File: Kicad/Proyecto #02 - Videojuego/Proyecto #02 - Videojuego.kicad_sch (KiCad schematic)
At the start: 16 parts

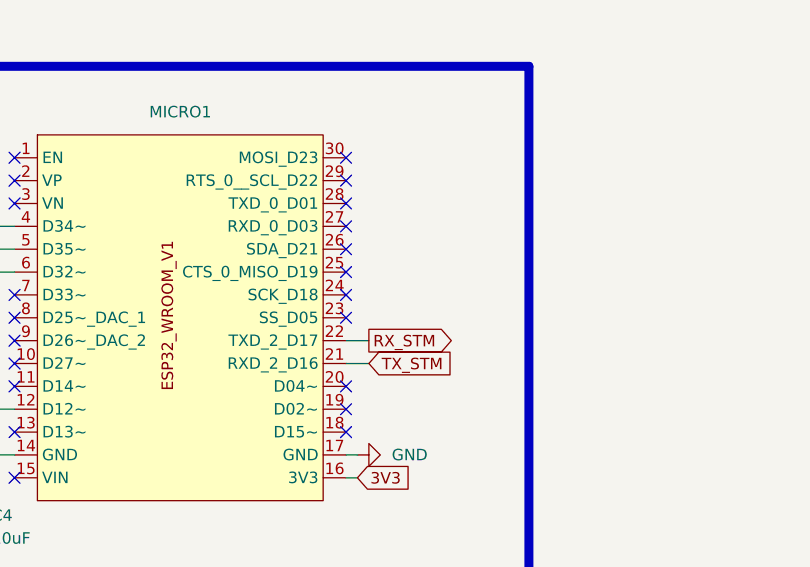
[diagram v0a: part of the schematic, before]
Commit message: A
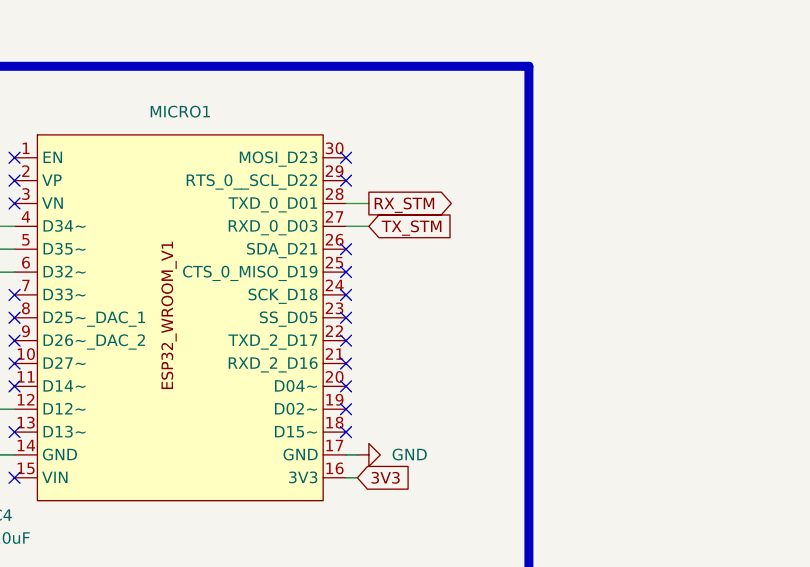
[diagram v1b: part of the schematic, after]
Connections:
- net RX_STM: now also MICRO1.28 (TXD_0_D01); no longer MICRO1.22 (TXD_2_D17)
- net TX_STM: now also MICRO1.27 (RXD_0_D03); no longer MICRO1.21 (RXD_2_D16)
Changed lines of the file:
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@@
-	)
-	(no_connect
-		(at 340.36 152.4)
 	)
 	(no_connect
@@
 	)
 	(no_connect
+		(at 340.36 170.18)
+	)
+	(no_connect
 		(at 193.04 54.61)
 	)
@@
 	)
 	(no_connect
+		(at 340.36 167.64)
+	)
+	(no_connect
 		(at 303.53 152.4)
 	)
@@
 	)
 	(no_connect
-		(at 340.36 154.94)
-	)
-	(no_connect
 		(at 193.04 50.8)
 	)
@@
 	(wire
 		(pts
-			(xy 340.36 167.64) (xy 342.9 167.64)
-		)
-		(stroke
-			(width 0)
-			(type default)
-		)
-	)
-	(wire
-		(pts
 			(xy 198.12 175.26) (xy 198.12 205.74)
 		)
@@
 	(wire
 		(pts
+			(xy 340.36 154.94) (xy 342.9 154.94)
+		)
+		(stroke
+			(width 0)
+			(type default)
+		)
+	)
+	(wire
+		(pts
 			(xy 205.74 152.4) (xy 205.74 213.36)
 		)
@@
 	(wire
 		(pts
+			(xy 340.36 152.4) (xy 342.9 152.4)
+		)
+		(stroke
+			(width 0)
+			(type default)
+		)
+	)
+	(wire
+		(pts
 			(xy 349.25 85.09) (xy 349.25 87.63)
 		)
@@
 		(pts
 			(xy 156.21 215.9) (xy 156.21 243.84)
-		)
-		(stroke
-			(width 0)
-			(type default)
-		)
-	)
-	(wire
-		(pts
-			(xy 340.36 170.18) (xy 342.9 170.18)
 		)
 		(stroke
@@
 	(global_label "RX_STM"
 		(shape output)
-		(at 342.9 167.64 0)
+		(at 342.9 152.4 0)
 		(fields_autoplaced yes)
 		(effects
@@
 		)
 		(property "Intersheetrefs" "${INTERSHEET_REFS}"
-			(at 352.8703 167.64 0)
+			(at 352.8703 152.4 0)
 			(effects
 				(font
@@
 	(global_label "TX_STM"
 		(shape input)
-		(at 342.9 170.18 0)
+		(at 342.9 154.94 0)
 		(fields_autoplaced yes)
 		(effects
@@
 		)
 		(property "Intersheetrefs" "${INTERSHEET_REFS}"
-			(at 352.673 170.18 0)
+			(at 352.673 154.94 0)
 			(effects
 				(font

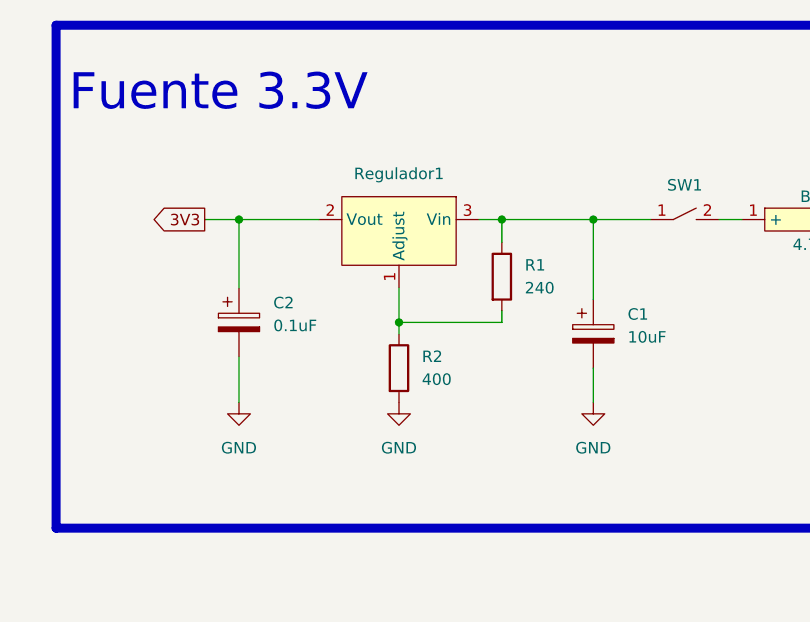
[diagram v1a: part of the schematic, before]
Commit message: A
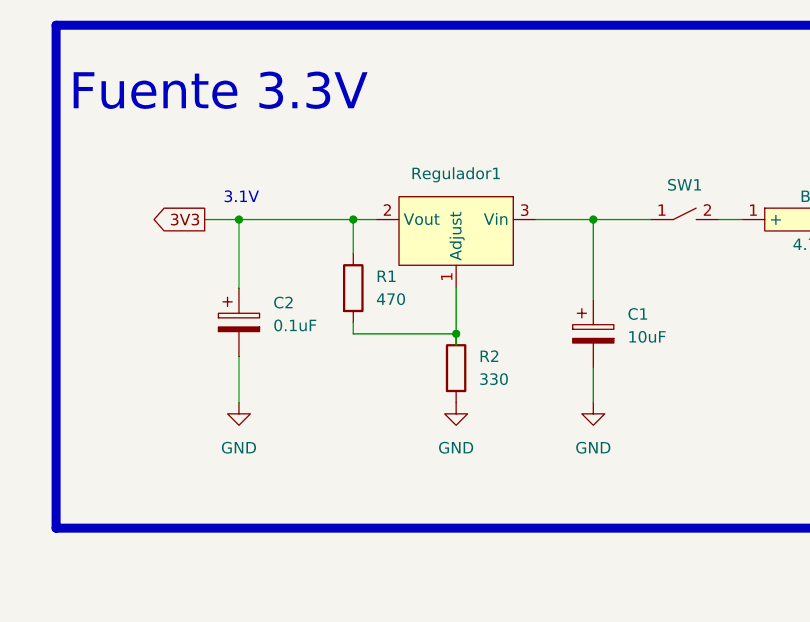
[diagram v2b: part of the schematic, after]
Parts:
- R1: value 240 -> 470
- R2: value 400 -> 330
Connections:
- net 3V3: now also R1.1
- net at C1.1, Regulador1.3 (Vin), SW1.1: no longer R1.1
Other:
- note added: "3.1V"
- moved on the sheet: R1, R2, Regulador1
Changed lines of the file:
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@@
-	)
-	(junction
-		(at 293.37 96.52)
-		(diameter 0)
-		(color 0 0 0 0)
 	)
 	(junction
@@
 	)
 	(junction
-		(at 297.18 175.26)
+		(at 299.72 97.79)
 		(diameter 0)
 		(color 0 0 0 0)
 	)
 	(junction
-		(at 304.8 85.09)
+		(at 297.18 175.26)
 		(diameter 0)
 		(color 0 0 0 0)
@@
 		(color 0 0 0 0)
 	)
+	(junction
+		(at 288.29 85.09)
+		(diameter 0)
+		(color 0 0 0 0)
+	)
 	(no_connect
 		(at 193.04 115.57)
@@
 	(wire
 		(pts
-			(xy 304.8 96.52) (xy 304.8 95.25)
-		)
-		(stroke
-			(width 0)
-			(type default)
-		)
-	)
-	(wire
-		(pts
 			(xy 153.67 213.36) (xy 153.67 238.76)
 		)
@@
 	(wire
 		(pts
-			(xy 304.8 85.09) (xy 314.96 85.09)
-		)
-		(stroke
-			(width 0)
-			(type default)
-		)
-	)
-	(wire
-		(pts
 			(xy 203.2 210.82) (xy 151.13 210.82)
 		)
@@
 	(wire
 		(pts
-			(xy 293.37 96.52) (xy 304.8 96.52)
-		)
-		(stroke
-			(width 0)
-			(type default)
-		)
-	)
-	(wire
-		(pts
 			(xy 115.57 233.68) (xy 118.11 233.68)
 		)
@@
 	(wire
 		(pts
-			(xy 293.37 92.71) (xy 293.37 96.52)
+			(xy 299.72 92.71) (xy 299.72 97.79)
 		)
 		(stroke
@@
 	(wire
 		(pts
+			(xy 288.29 85.09) (xy 290.83 85.09)
+		)
+		(stroke
+			(width 0)
+			(type default)
+		)
+	)
+	(wire
+		(pts
 			(xy 328.93 85.09) (xy 331.47 85.09)
 		)
@@
 	(wire
 		(pts
-			(xy 293.37 96.52) (xy 293.37 97.79)
-		)
-		(stroke
-			(width 0)
-			(type default)
-		)
-	)
-	(wire
-		(pts
 			(xy 193.04 186.69) (xy 194.31 186.69)
 		)
@@
 	(wire
 		(pts
-			(xy 302.26 85.09) (xy 304.8 85.09)
+			(xy 308.61 85.09) (xy 314.96 85.09)
 		)
 		(stroke
@@
 	(wire
 		(pts
+			(xy 288.29 97.79) (xy 299.72 97.79)
+		)
+		(stroke
+			(width 0)
+			(type default)
+		)
+	)
+	(wire
+		(pts
 			(xy 203.2 160.02) (xy 203.2 210.82)
 		)
@@
 	(wire
 		(pts
+			(xy 288.29 97.79) (xy 288.29 96.52)
+		)
+		(stroke
+			(width 0)
+			(type default)
+		)
+	)
+	(wire
+		(pts
+			(xy 299.72 99.06) (xy 299.72 97.79)
+		)
+		(stroke
+			(width 0)
+			(type default)
+		)
+	)
+	(wire
+		(pts
 			(xy 67.31 167.64) (xy 69.85 167.64)
 		)
@@
 	(wire
 		(pts
+			(xy 288.29 88.9) (xy 288.29 85.09)
+		)
+		(stroke
+			(width 0)
+			(type default)
+		)
+	)
+	(wire
+		(pts
 			(xy 64.77 220.98) (xy 118.11 220.98)
 		)
@@
 	(wire
 		(pts
-			(xy 304.8 87.63) (xy 304.8 85.09)
-		)
-		(stroke
-			(width 0)
-			(type default)
-		)
-	)
-	(wire
-		(pts
 			(xy 68.58 213.36) (xy 118.11 213.36)
 		)
@@
 	(wire
 		(pts
-			(xy 275.59 85.09) (xy 284.48 85.09)
+			(xy 275.59 85.09) (xy 288.29 85.09)
 		)
 		(stroke
@@
 		(fill
 			(type none)
+		)
+	)
+	(text "3.1V\n"
+		(exclude_from_sim no)
+		(at 275.844 82.804 0)
+		(effects
+			(font
+				(size 1.27 1.27)
+			)
 		)
 	)
@@
 	(symbol
 		(lib_id "Device:R")
-		(at 304.8 91.44 0)
+		(at 288.29 92.71 0)
 		(unit 1)
 		(exclude_from_sim no)
@@
 		(fields_autoplaced yes)
 		(property "Reference" "R1"
-			(at 307.34 90.17 0)
+			(at 290.83 91.44 0)
 			(effects
 				(font
@@
 			)
 		)
-		(property "Value" "240"
-			(at 307.34 92.71 0)
+		(property "Value" "470"
+			(at 290.83 93.98 0)
 			(effects
 				(font
@@
 		)
 		(property "Footprint" ""
-			(at 303.022 91.44 90)
+			(at 286.512 92.71 90)
 			(effects
 				(font
@@
 		)
 		(property "Datasheet" "~"
-			(at 304.8 91.44 0)
+			(at 288.29 92.71 0)
 			(effects
 				(font
@@
 		)
 		(property "Description" "Resistor"
-			(at 304.8 91.44 0)
+			(at 288.29 92.71 0)
 			(effects
 				(font
@@
 	(symbol
 		(lib_id "Device:R")
-		(at 293.37 101.6 0)
+		(at 299.72 101.6 0)
 		(unit 1)
 		(exclude_from_sim no)
@@
 		(fields_autoplaced yes)
 		(property "Reference" "R2"
-			(at 295.91 100.33 0)
+			(at 302.26 100.33 0)
 			(effects
 				(font
@@
 			)
 		)
-		(property "Value" "400"
-			(at 295.91 102.87 0)
+		(property "Value" "330"
+			(at 302.26 102.87 0)
 			(effects
 				(font
@@
 		)
 		(property "Footprint" ""
-			(at 291.592 101.6 90)
+			(at 297.942 101.6 90)
 			(effects
 				(font
@@
 		)
 		(property "Datasheet" "~"
-			(at 293.37 101.6 0)
+			(at 299.72 101.6 0)
 			(effects
 				(font
@@
 		)
 		(property "Description" "Resistor"
-			(at 293.37 101.6 0)
+			(at 299.72 101.6 0)
 			(effects
 				(font
@@
 	(symbol
 		(lib_id "power:GND")
-		(at 293.37 105.41 0)
+		(at 299.72 105.41 0)
 		(unit 1)
 		(exclude_from_sim no)
@@
 		(fields_autoplaced yes)
 		(property "Reference" "#PWR05"
-			(at 293.37 111.76 0)
+			(at 299.72 111.76 0)
 			(effects
 				(font
@@
 		)
 		(property "Value" "GND"
-			(at 293.37 110.49 0)
+			(at 299.72 110.49 0)
 			(effects
 				(font
@@
 		)
 		(property "Footprint" ""
-			(at 293.37 105.41 0)
+			(at 299.72 105.41 0)
 			(effects
 				(font
@@
 		)
 		(property "Datasheet" ""
-			(at 293.37 105.41 0)
+			(at 299.72 105.41 0)
 			(effects
 				(font
@@
 		)
 		(property "Description" "Power symbol creates a global label with name \"GND\" , ground"
-			(at 293.37 105.41 0)
+			(at 299.72 105.41 0)
 			(effects
 				(font
@@
 	(symbol
 		(lib_id "JOYSTICK_KY-023:LM317")
-		(at 293.37 81.28 0)
+		(at 299.72 81.28 0)
 		(mirror y)
 		(unit 1)
@@
 		(dnp no)
 		(property "Reference" "Regulador1"
-			(at 293.37 80.01 0)
+			(at 299.72 80.01 0)
 			(effects
 				(font
@@
 		)
 		(property "Value" "~"
-			(at 293.37 81.28 0)
+			(at 299.72 81.28 0)
 			(effects
 				(font
@@
 		)
 		(property "Footprint" ""
-			(at 293.37 81.28 0)
+			(at 299.72 81.28 0)
 			(effects
 				(font
@@
 		)
 		(property "Datasheet" ""
-			(at 293.37 81.28 0)
+			(at 299.72 81.28 0)
 			(effects
 				(font
@@
 		)
 		(property "Description" ""
-			(at 293.37 81.28 0)
-			(effects
-				(font
+			(at 299.72 81.28 0)
+			(effects
+				(font

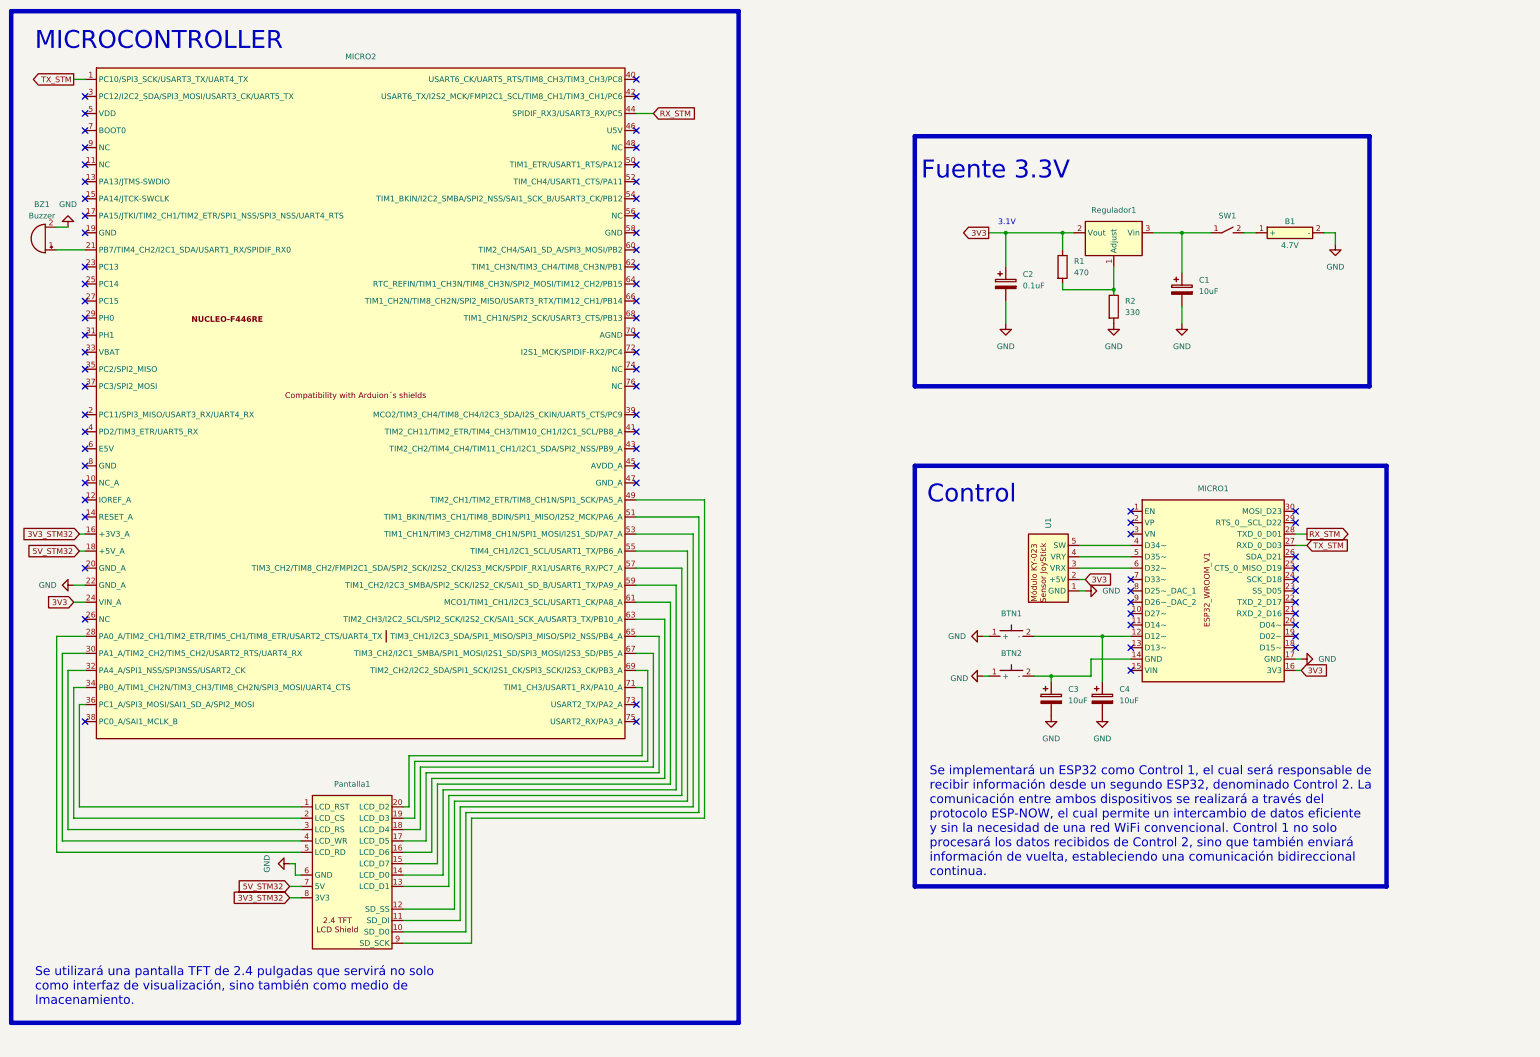
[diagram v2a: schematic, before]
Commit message: A
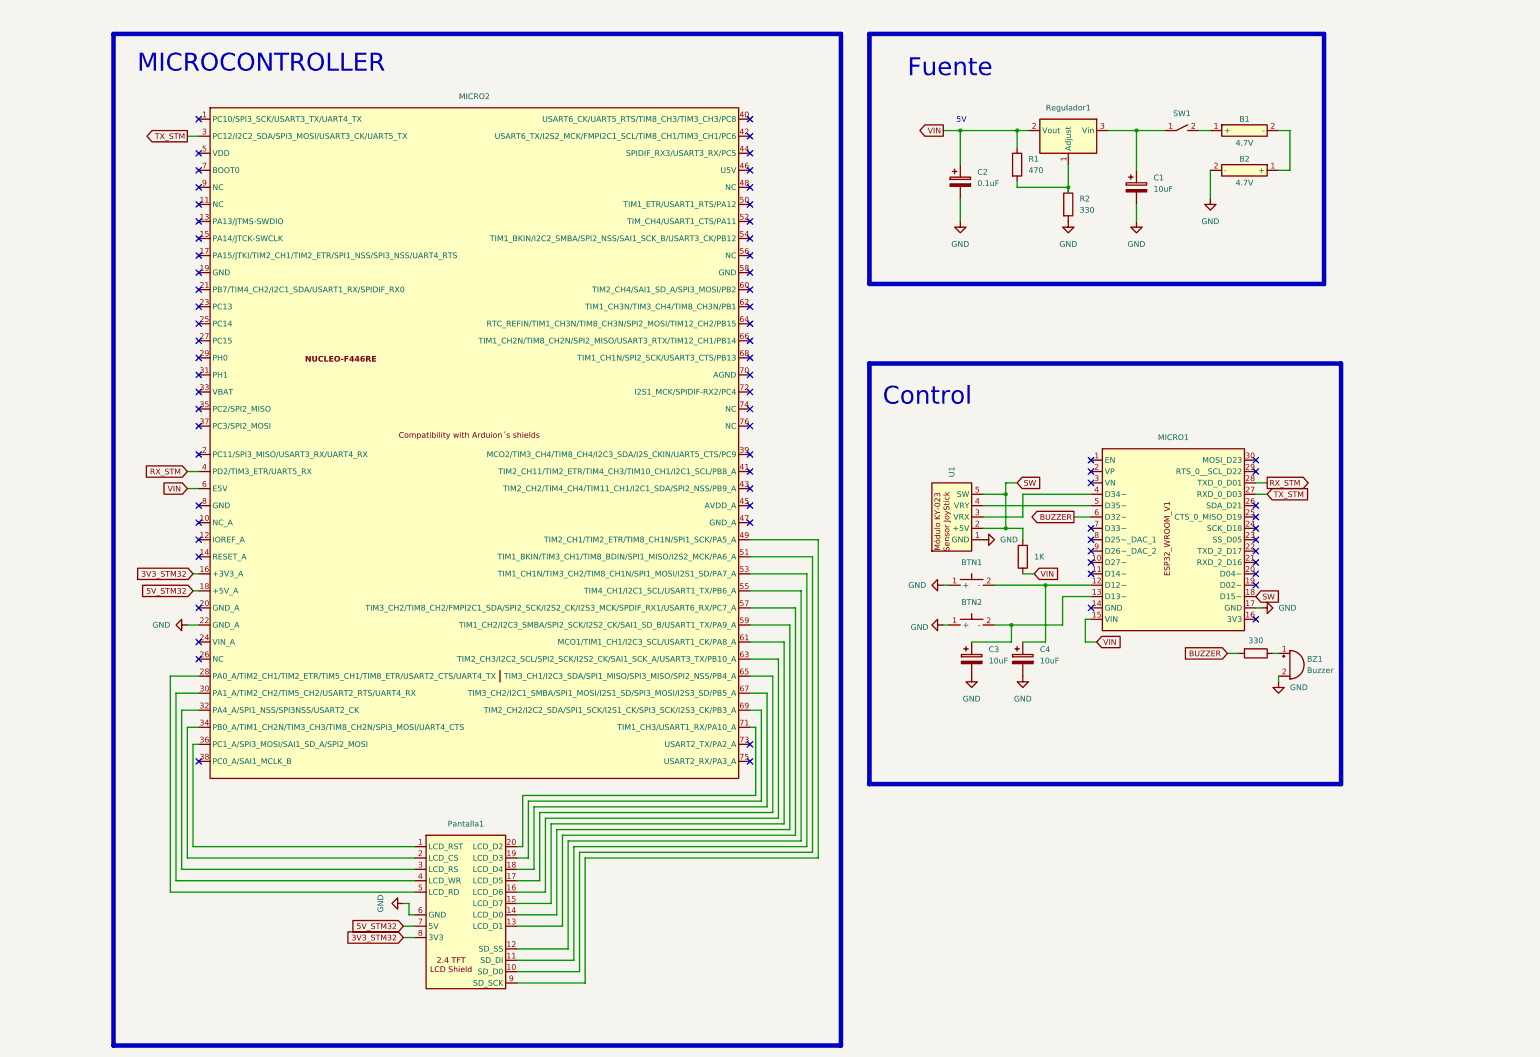
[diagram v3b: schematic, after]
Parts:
- added B2: 4.7V, symbol JOYSTICK_KY-023:Batterias
- added R3: 1K, symbol Device:R
- added R4: 330, symbol Device:R
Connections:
- net GND: now also B2.2 (-); no longer B1.2 (-)
- net RX_STM: now also MICRO2.4 (PD2/TIM3_ETR/UART5_RX); no longer MICRO2.44 (SPIDIF_RX3/USART3_RX/PC5)
- net TX_STM: now also MICRO2.3 (PC12/I2C2_SDA/SPI3_MOSI/USART3_CK/UART5_TX); no longer MICRO2.1 (PC10/SPI3_SCK/USART3_TX/UART4_TX)
- net at BTN2.2 (-), C3.1: now also MICRO1.13 (D13~); no longer MICRO1.14 (GND)
- net at BZ1.1 (+): now also R4.1; no longer MICRO2.21 (PB7/TIM4_CH2/I2C1_SDA/USART1_RX/SPIDIF_RX0)
- net VIN: now reaches MICRO1.15 (VIN)
- net VIN: now also C2.1, MICRO2.6 (E5V), R1.1, Regulador1.2 (Vout), R3.1
- net SW: now reaches MICRO1.18 (D15~)
- net SW: now also U1.2 (+5V), U1.5 (SW), R3.2
- net at MICRO1.4 (D34~): now also U1.3 (VRX); no longer U1.5 (SW)
- net BUZZER: now reaches MICRO1.6 (D32~)
- net BUZZER: now also R4.2; no longer U1.3 (VRX)
- removed net 3V3: C2.1, MICRO1.16 (3V3), MICRO2.24 (VIN_A), R1.1, Regulador1.2 (Vout), U1.2 (+5V)
- new net: B1.2 (-), B2.1 (+)
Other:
- note added: "5V"
- note added: "Fuente"
- note removed: "3.1V"
- note removed: "Fuente 3.3V"
- note removed: "Se implementará un ESP32 como Control 1, el cual será responsable de recibir información desde un segundo ESP32, denominado Control 2. La comunicación entre ambos dispositivos se realizará a través del protocolo ESP-NOW, el cual permite un intercambio de datos eficiente y sin la necesidad de una red WiFi convencional. Control 1 no solo procesará los datos recibidos de Control 2, sino que también 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"
- note removed: "Se utilizará una pantalla TFT de 2.4 pulgadas que servirá no solo como interfaz de visualización, sino también como medio de lmacenamiento."
- moved on the sheet: B1, BTN1, BTN2, BZ1, C1, C2, C3, C4, MICRO1, MICRO2, Pantalla1, R1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
